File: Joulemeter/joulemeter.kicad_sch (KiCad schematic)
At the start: 13 parts, among them J1 XT60-M, J2 XT60-M, J3 22035035, U2 INA240A1PW, U5 PADS131M04QPWRQ1

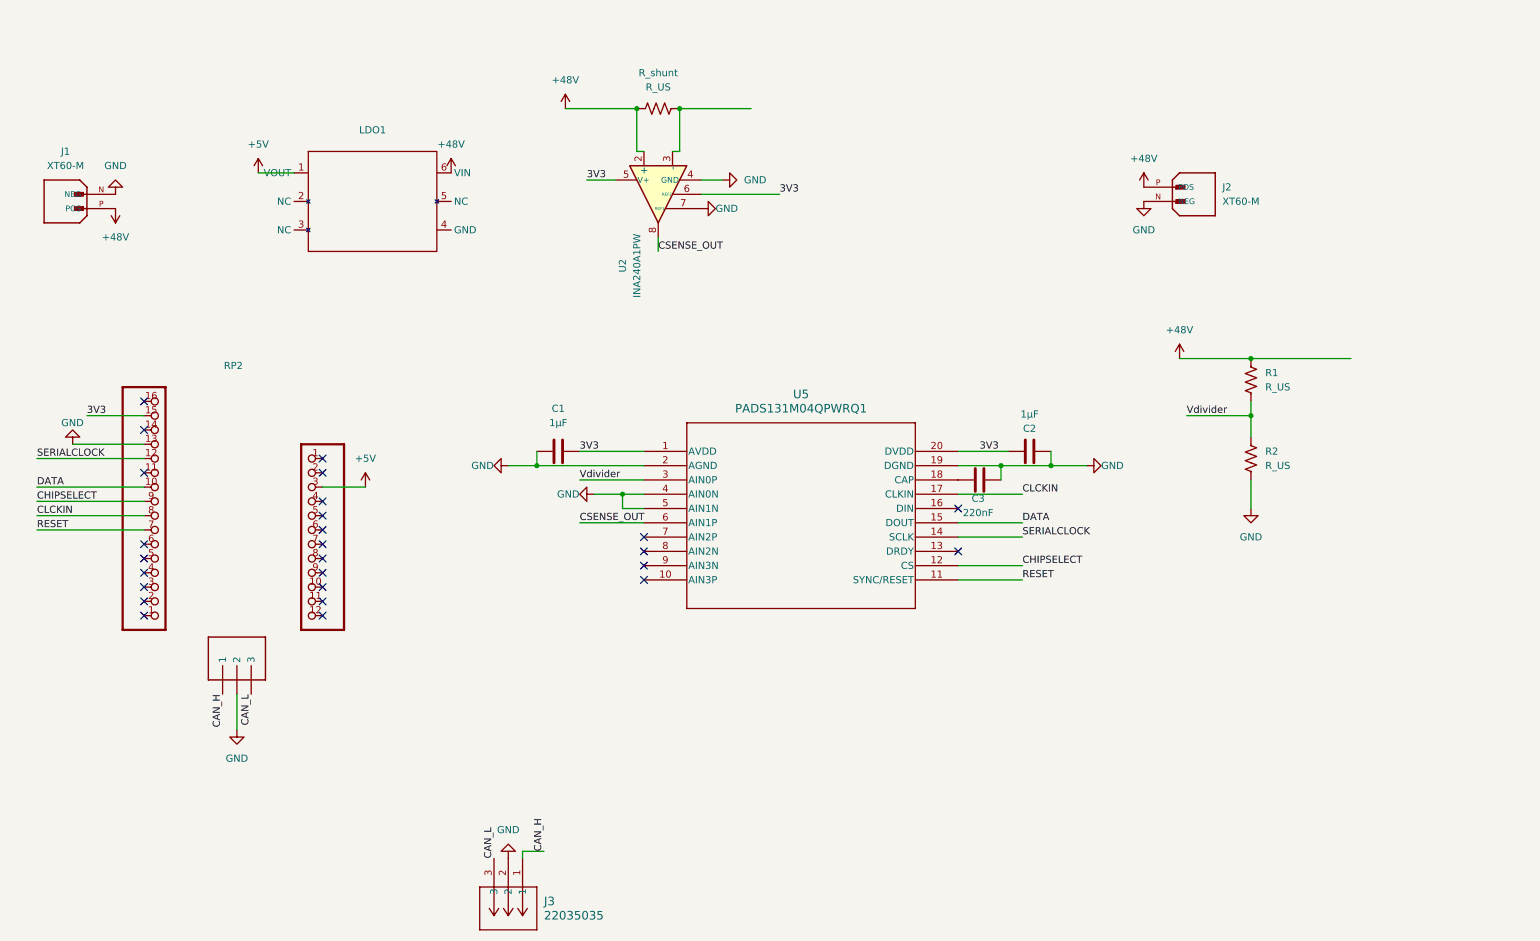
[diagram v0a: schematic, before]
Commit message: schematic feedback
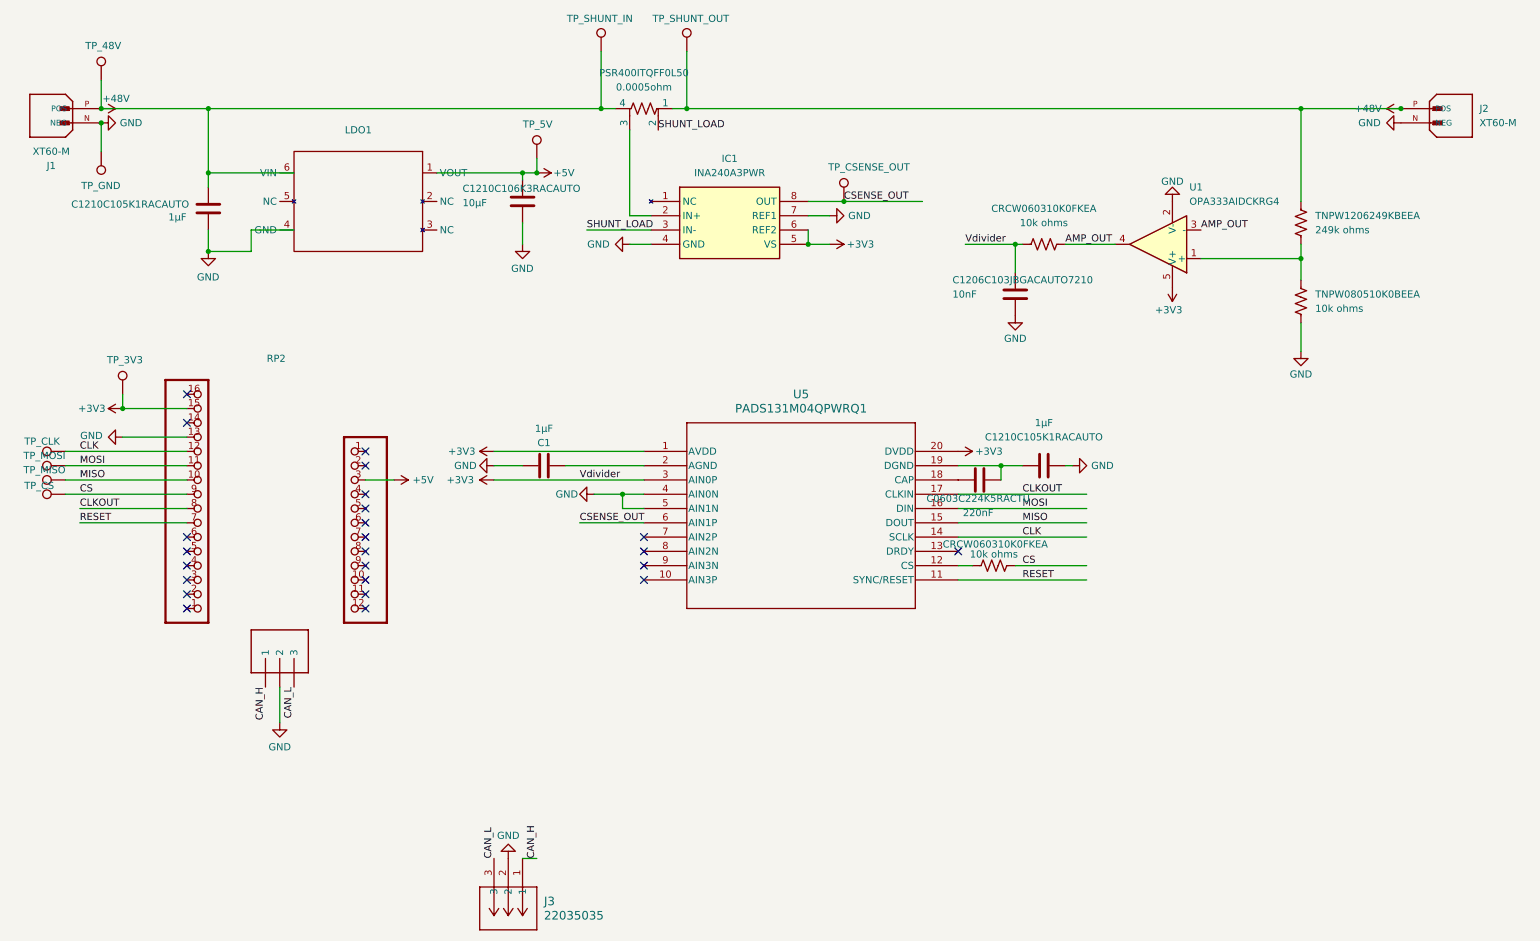
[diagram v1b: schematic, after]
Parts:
- removed R_shunt: R_US, symbol Device:R_US
- removed U2: INA240A1PW, Package_SO:TSSOP-8_4.4x3mm_P0.65mm, symbol Amplifier_Current:INA240A1PW
- added C1206C103JBGACAUTO7210: 10nF, symbol Device:C
- added C1210C105K1RACAUTO: 1μF, symbol Device:C
- added C1210C106K3RACAUTO: 10μF, symbol Device:C
- added CRCW060310K0FKEA (x2): 10k ohms, symbol Device:R_US
- added IC1: INA240A3PWR, SOP65P640X120-8N, symbol INA240A3PWR:INA240A3PWR
- added PSR400ITQFF0L50: 0.0005ohm, symbol Device:R_Shunt_US
- added TP_3V3, TP_48V, TP_5V, TP_CLK, TP_CS, TP_CSENSE_OUT, TP_GND, TP_MISO, TP_MOSI, TP_SHUNT_IN, TP_SHUNT_OUT: ~, symbol Connector:TestPoint
- added U1: OPA333AIDCKRG4, Package_TO_SOT_SMD:SOT-353_SC-70-5, symbol Amplifier_Operational:OPA333xxDCK
- TNPW080510K0BEEA: renamed from R2; value R_US -> 10k ohms
- TNPW1206249KBEEA: renamed from R1; value R_US -> 249k ohms
- renumbered C3 to C0603C224K5RACTU, C2 to C1210C105K1RACAUTO
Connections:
- net CLCKIN is gone; now on net CLKOUT: RP2.8, U5.17 (CLKIN)
- net DATA is gone; now on net MISO: RP2.10, U5.15 (DOUT)
- net SERIALCLOCK is gone; now on net CLK: RP2.12, U5.14 (SCLK)
- net +48V: now also LDO1.6 (VIN), C1210C105K1RACAUTO.1, PSR400ITQFF0L50.1, PSR400ITQFF0L50.4, TP_48V.1, TP_SHUNT_IN.1, TP_SHUNT_OUT.1
- net +5V: now also C1210C106K3RACAUTO.1, TP_5V.1
- net CSENSE_OUT: now also IC1.8 (OUT), TP_CSENSE_OUT.1
- net GND: now also C1.1, LDO1.4 (GND), C1206C103JBGACAUTO7210.2, C1210C105K1RACAUTO.2, C1210C106K3RACAUTO.2, IC1.4 (GND), IC1.7 (REF1), TP_GND.1, U1.2 (V-); no longer C0603C224K5RACTU.2, C1.2, U5.19 (DGND), U5.2 (AGND)
- net MISO: now reaches RP2.10
- net MISO: now also TP_MISO.1
- net MOSI: now reaches RP2.11
- net MOSI: now also U5.16 (DIN), TP_MOSI.1
- net CLK: now reaches RP2.12
- net CLK: now also TP_CLK.1
- net CLKOUT: now reaches RP2.8
- net CS: now reaches RP2.9
- net CS: now also CRCW060310K0FKEA.2, TP_CS.1
- net 3V3 renamed +3V3
- net +3V3: now also U5.3 (AIN0P), C1206C103JBGACAUTO7210.1, CRCW060310K0FKEA.1, IC1.5 (VS), IC1.6 (REF2), TP_3V3.1, U1.5 (V+); no longer C1.1, C1210C105K1RACAUTO.1
- net CHIPSELECT: no longer names the net of U5.12 (CS)
- net CHIPSELECT: now also CRCW060310K0FKEA.1; no longer RP2.9
- net Vdivider: no longer names the net of TNPW080510K0BEEA.1, TNPW1206249KBEEA.2
- net Vdivider: now also U1.1 (+); no longer U5.3 (AIN0P)
- new net: IC1.2 (IN+), PSR400ITQFF0L50.3
- new net: C1.2, U5.2 (AGND)
- new net: C0603C224K5RACTU.2, C1210C105K1RACAUTO.1, U5.19 (DGND)
- new net AMP_OUT: CRCW060310K0FKEA.2, U1.3 (-), U1.4
- new net SHUNT_LOAD: IC1.3 (IN-), PSR400ITQFF0L50.2
- no-connect marks 26 -> 24
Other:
- moved on the sheet: C1210C105K1RACAUTO, J1, J2, LDO1, RP2, TNPW080510K0BEEA, TNPW1206249KBEEA
